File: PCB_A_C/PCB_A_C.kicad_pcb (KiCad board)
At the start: 2 copper layers, 18 parts, among them J1 Conn_01x08_Socket, J2 Conn_01x04, J3 Screw_Terminal_01x02, SW1 SW_Push, SW2 SW_Push, SW3 SW_Push, SW4 SW_Push, SW5 SW_Push, U1 DHT11, U2 MSP430G2553IN20, Y0 32kHz

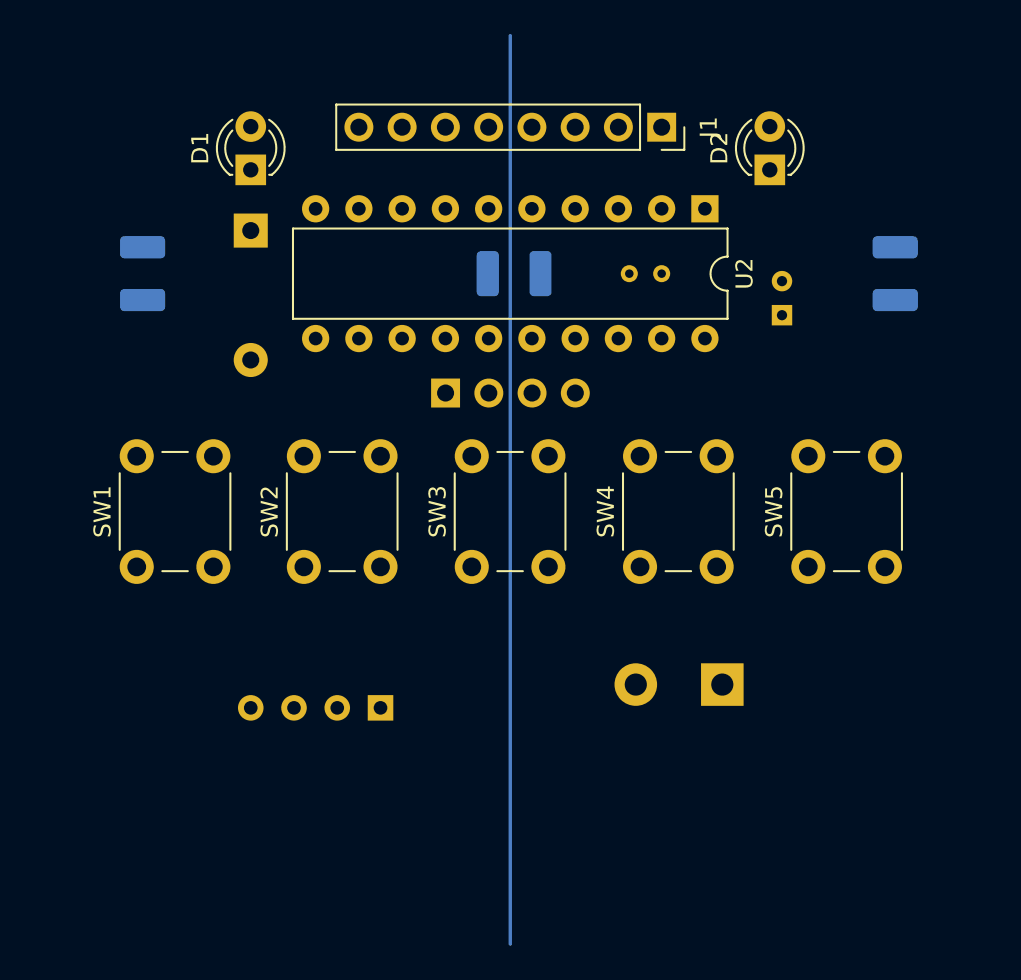
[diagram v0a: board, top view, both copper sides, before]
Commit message: Routed PCB.
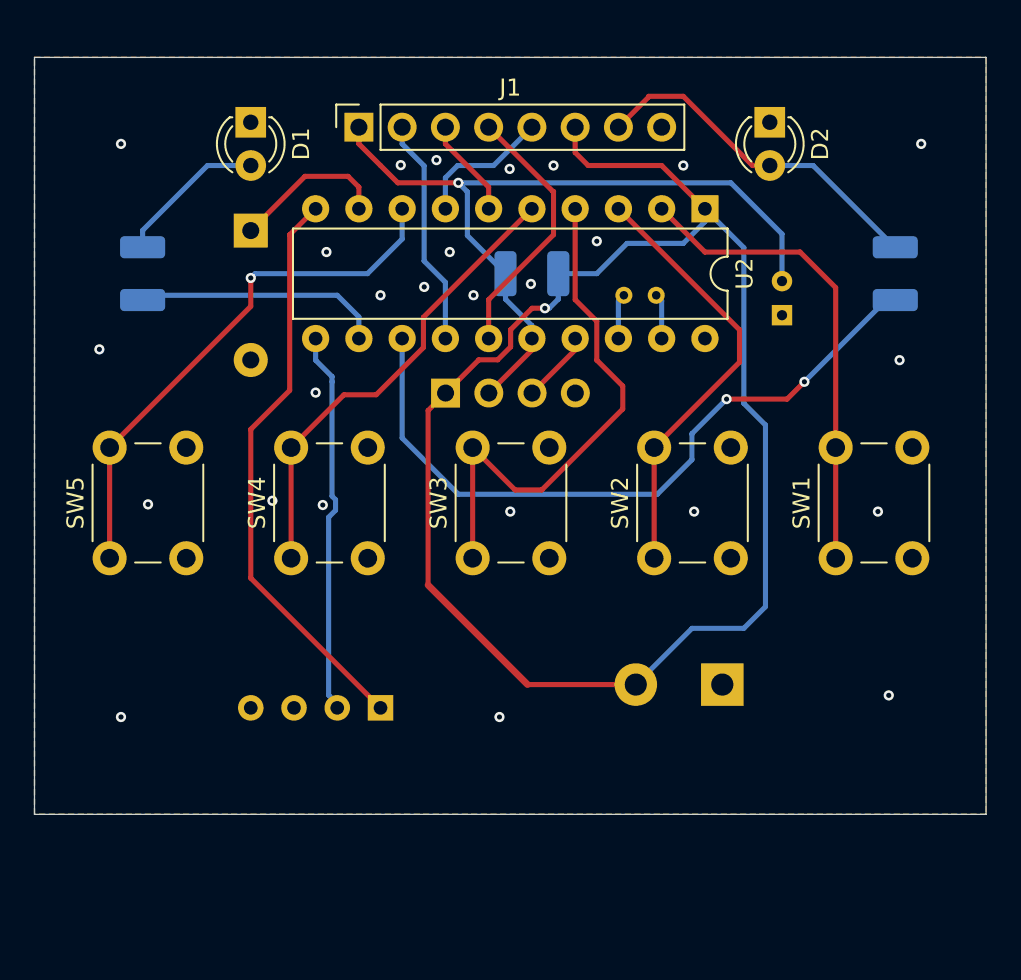
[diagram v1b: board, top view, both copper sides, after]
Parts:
- J1: value Conn_01x08_Socket -> Conn01x08
- moved SW1 41.0 mm to (171.5, 104.3)
- moved SW5 41.0 mm to (128.9, 104.3)
- moved SW2 20.6 mm to (160.8, 104.3)
- moved SW4 20.5 mm to (139.5, 104.3)
- moved J1 17.8 mm to (143.5, 79.0), turned to 90 degrees
- moved D1 2.79 mm to (137.2, 78.7), turned to -90 degrees
- moved D2 2.79 mm to (167.6, 78.7), turned to -90 degrees
- moved Y0 1.31 mm to (161.0, 88.9)
- moved R1 1.04 mm to (153.7, 87.6), turned to 180 degrees
- moved SW3 0.51 mm to (150.2, 104.3)
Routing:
- net +BATT: track 0.00 -> 93.1 mm, vias 0 -> 1
- net RST: track 0.00 -> 46.6 mm, vias 0 -> 1
- net Net-(U2-P2.5/TA1.2): track 0.00 -> 41.8 mm, vias 0 -> 2
- net P2.2: track 0.00 -> 34.0 mm
- net P2.0: track 0.00 -> 31.8 mm, vias 0 -> 1
- net Net-(U2-UCA0TXD/UCA0SIMO/TA0.1/CA2/A2/P1.2): track 0.00 -> 31.2 mm
- net Net-(U2-TA0CLK/ACLK/CA0/A0/P1.0): track 0.00 -> 28.0 mm
- net Net-(U2-CAOUT/VREF-/VeREF-/CA3/A3/P1.3): track 0.00 -> 27.5 mm
- net Net-(U2-UCA0RXD/UCA0SOMI/TA0.0/CA1/A1/P1.1): track 0.00 -> 25.5 mm
- net P2.3: track 0.00 -> 22.7 mm
- net LIGHT: track 0.00 -> 20.7 mm
- net DIN: track 0.00 -> 15.6 mm
- net Net-(U2-P2.4/TA1.2): track 0.00 -> 14.6 mm
- net CE: track 0.00 -> 13.5 mm
- net Net-(BZ1--): track 0.00 -> 9.20 mm
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- added copper zone on B.Cu, net -BATT
- added copper zone on F.Cu, net -BATT
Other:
- board outline added: 55.9 x 44.4 mm
